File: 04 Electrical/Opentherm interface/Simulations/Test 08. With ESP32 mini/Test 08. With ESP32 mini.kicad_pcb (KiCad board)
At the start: 2 copper layers, 79 x 36 mm, 29 parts, among them J1 OpenTherm, J2 Laser range sensor, J3 ST7789, J4 Encoder, Q1 MMBT2907A, U1 DS18S20, U2 DS18S20, U3 DS18S20, U4 DS18S20, U5 EL357N-G, U6 EL357N-G, U7 mini_esp32

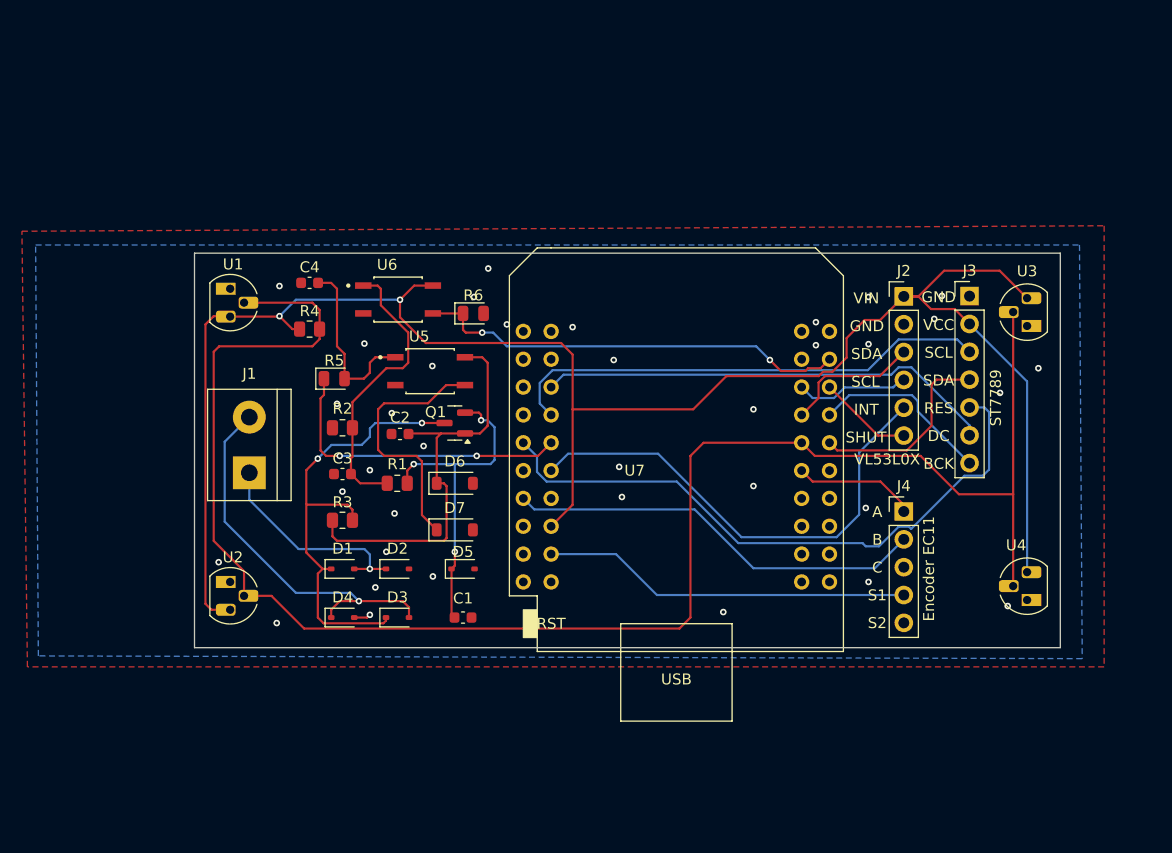
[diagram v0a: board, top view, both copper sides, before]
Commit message: mch
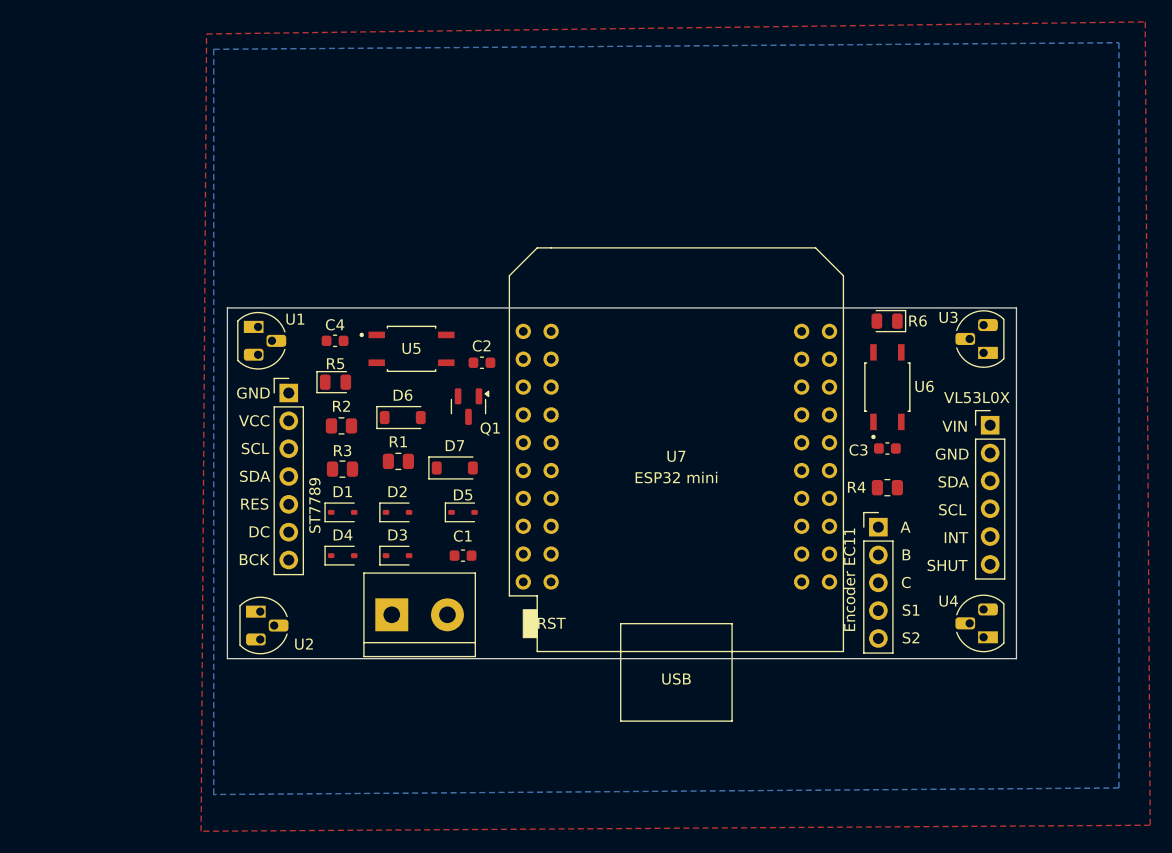
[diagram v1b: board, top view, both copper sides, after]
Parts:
- moved J3 62.7 mm to (98.6, 82.8)
- moved R4 54.7 mm to (153.2, 91.4)
- moved C3 49.8 mm to (153.2, 87.8), turned to 180 degrees
- moved U6 45.4 mm to (153.2, 82.2), turned to 90 degrees
- moved R6 37.8 mm to (153.2, 76.2), turned to 180 degrees
- moved J1 18.4 mm to (108.0, 103.0), turned to 0 degrees
- moved J2 14.2 mm to (162.6, 85.7)
- moved C2 9.91 mm to (116.2, 80.0)
- moved D6 7.65 mm to (109.0, 85.0)
- moved C4 5.78 mm to (102.8, 78.0)
- moved C1 5.65 mm to (114.5, 97.6)
- moved D3 5.65 mm to (108.5, 97.6)
- moved D4 5.65 mm to (103.5, 97.6)
- moved D7 5.65 mm to (113.8, 89.6)
- moved U4 5.23 mm to (162.0, 105.0)
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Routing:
- net +3V3: track 168.4 -> 0.00 mm, vias 2 -> 0
- net onewire: track 157.4 -> 0.00 mm
- net Disp_RES: track 57.5 -> 0.00 mm
- net Disp_SCK: track 44.7 -> 0.00 mm
- net TOF_INT: track 44.2 -> 0.00 mm
- net Disp_DC: track 42.0 -> 0.00 mm
- net Net-(D1-K): track 41.9 -> 0.00 mm, vias 2 -> 0
- net cntr_to_boil: track 39.7 -> 0.00 mm, vias 2 -> 0
- net Enc_B: track 38.4 -> 0.00 mm
- net Net-(D6-K): track 38.2 -> 0.00 mm
- net Net-(D3-A): track 35.0 -> 0.00 mm, vias 1 -> 0
- net Enc_S: track 33.7 -> 0.00 mm
- net Net-(D5-K): track 30.3 -> 0.00 mm, vias 3 -> 0
- net boil_to_cntr: track 28.4 -> 0.00 mm, vias 2 -> 0
- net Net-(C3-Pad2): track 26.4 -> 0.00 mm
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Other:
- board size 79 x 36 mm -> 72 x 32 mm
- board text added: "ESP32 mini"
